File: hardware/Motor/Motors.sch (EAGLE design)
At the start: 34 parts, among them IC1 MC33269ST, Q1 BSS138, Q2 BSS138, U1 DRV8884PWPR, U2 PHOTON_WITH_HEADERS, U3 LS7083N-S

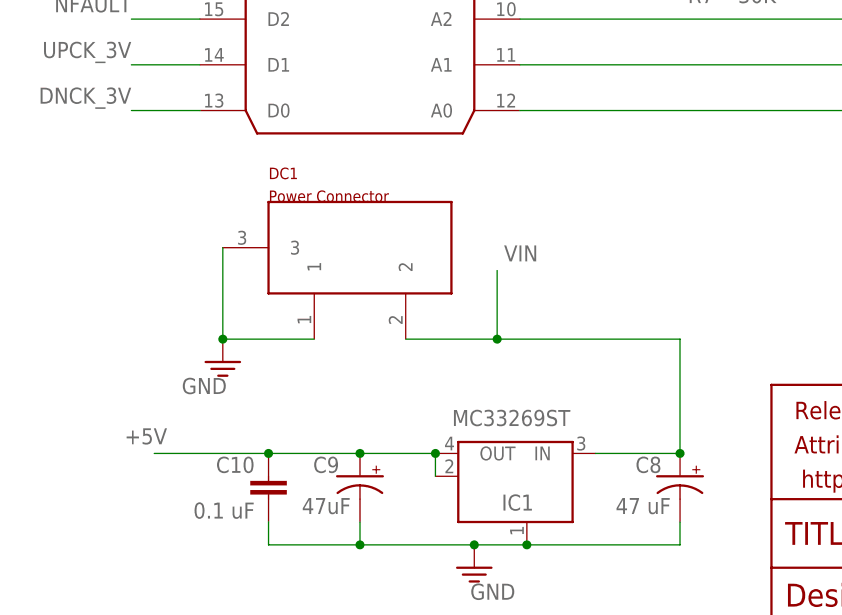
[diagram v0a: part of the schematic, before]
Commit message: Cumulative changes: adding light sources, boards, firmwares, construction details
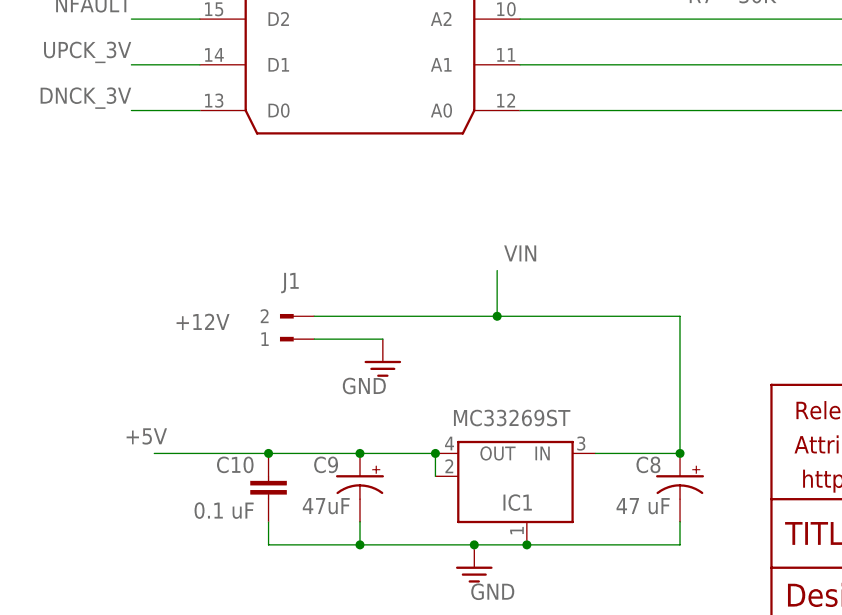
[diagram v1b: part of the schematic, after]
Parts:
- removed DC1: Power Connector, Spectron2:POWERSUPPLY_DC21MMX
- added J1: +12V, WEIDMULLER-PM5.08_2_90BLK:PM5.08/2/90BLK
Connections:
- net GND: now also J1.1; no longer DC1.1, DC1.3
- net VIN: now also J1.2; no longer DC1.2
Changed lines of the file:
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@@
 <?xml version="1.0" encoding="utf-8"?>
 <!DOCTYPE eagle SYSTEM "eagle.dtd">
-<eagle version="7.7.0">
+<eagle version="8.0.1">
 <drawing>
 <settings>
@@
 <layers>
 <layer number="1" name="Top" color="4" fill="1" visible="no" active="no"/>
+<layer number="2" name="Route2" color="1" fill="3" visible="no" active="no"/>
+<layer number="3" name="Route3" color="4" fill="3" visible="no" active="no"/>
+<layer number="4" name="Route4" color="1" fill="4" visible="no" active="no"/>
+<layer number="5" name="Route5" color="4" fill="4" visible="no" active="no"/>
+<layer number="6" name="Route6" color="1" fill="8" visible="no" active="no"/>
+<layer number="7" name="Route7" color="4" fill="8" visible="no" active="no"/>
+<layer number="8" name="Route8" color="1" fill="2" visible="no" active="no"/>
+<layer number="9" name="Route9" color="4" fill="2" visible="no" active="no"/>
+<layer number="10" name="Route10" color="1" fill="7" visible="no" active="no"/>
+<layer number="11" name="Route11" color="4" fill="7" visible="no" active="no"/>
+<layer number="12" name="Route12" color="1" fill="5" visible="no" active="no"/>
+<layer number="13" name="Route13" color="4" fill="5" visible="no" active="no"/>
+<layer number="14" name="Route14" color="1" fill="6" visible="no" active="no"/>
+<layer number="15" name="Route15" color="4" fill="6" visible="no" active="no"/>
 <layer number="16" name="Bottom" color="1" fill="1" visible="no" active="no"/>
 <layer number="17" name="Pads" color="2" fill="1" visible="no" active="no"/>
@@
 <part name="U2" library="Spectron2" deviceset="PHOTON" device="_WITH_HEADERS"/>
 <part name="U1" library="TI-DRV8884" deviceset="DRV8884PWPR" device=""/>
-<part name="DC1" library="Spectron2" deviceset="POWERSUPPLY_DC21MM" device="X" value="Power Connector"/>
 <part name="GND1" library="Spectron2" deviceset="GND" device=""/>
 <part name="GND6" library="Spectron2" deviceset="GND" device=""/>
@@
 <part name="GND10" library="Spectron2" deviceset="GND" device=""/>
 <part name="R7" library="Spectron2" deviceset="R-EU_" device="R0805" value="30K"/>
+<part name="J1" library="WEIDMULLER-PM5.08_2_90BLK" deviceset="PM5.08/2/90BLK" device="" value="+12V"/>
 </parts>
 <sheets>
@@
 <instance part="U2" gate="G$1" x="33.02" y="30.48" rot="MR0"/>
 <instance part="U1" gate="A" x="137.16" y="25.4"/>
-<instance part="DC1" gate="G$1" x="33.02" y="-12.7"/>
 <instance part="GND1" gate="1" x="119.38" y="2.54" rot="MR0"/>
-<instance part="GND6" gate="1" x="17.78" y="-25.4"/>
+<instance part="GND6" gate="1" x="35.56" y="-25.4"/>
 <instance part="IC1" gate="G$1" x="51.562" y="-40.64" smashed="yes" rot="MR0">
 <attribute name="NAME" x="52.324" y="-41.91" size="1.778" layer="95" rot="MR0"/>
@@
 <attribute name="VALUE" x="79.248" y="16.256" size="1.778" layer="96" rot="R180"/>
 </instance>
+<instance part="J1" gate="A" x="27.94" y="-22.86" smashed="yes" rot="R180">
+<attribute name="NAME" x="26.416" y="-15.494" size="1.778" layer="95" rot="R180"/>
+<attribute name="VALUE" x="18.542" y="-20.066" size="1.778" layer="96" rot="R180"/>
+</instance>
 </instances>
 <busses>
@@
 <net name="VIN" class="0">
 <segment>
-<wire x1="38.1" y1="-22.86" x2="48.26" y2="-22.86" width="0.1524" layer="91"/>
-<pinref part="DC1" gate="G$1" pin="2"/>
-<wire x1="48.26" y1="-22.86" x2="48.26" y2="-15.24" width="0.1524" layer="91"/>
+<wire x1="48.26" y1="-20.32" x2="48.26" y2="-15.24" width="0.1524" layer="91"/>
 <label x="49.022" y="-14.224" size="1.778" layer="95"/>
 <pinref part="IC1" gate="G$1" pin="IN"/>
 <pinref part="C8" gate="G$1" pin="+"/>
 <wire x1="68.58" y1="-35.56" x2="59.182" y2="-35.56" width="0.1524" layer="91"/>
-<wire x1="68.58" y1="-35.56" x2="68.58" y2="-22.86" width="0.1524" layer="91"/>
-<wire x1="68.58" y1="-22.86" x2="48.26" y2="-22.86" width="0.1524" layer="91"/>
+<wire x1="68.58" y1="-35.56" x2="68.58" y2="-20.32" width="0.1524" layer="91"/>
+<wire x1="68.58" y1="-20.32" x2="48.26" y2="-20.32" width="0.1524" layer="91"/>
 <junction x="68.58" y="-35.56"/>
-<junction x="48.26" y="-22.86"/>
+<junction x="48.26" y="-20.32"/>
+<pinref part="J1" gate="A" pin="2"/>
+<wire x1="27.94" y1="-20.32" x2="48.26" y2="-20.32" width="0.1524" layer="91"/>
 </segment>
 <segment>
@@
 </segment>
 <segment>
-<pinref part="DC1" gate="G$1" pin="3"/>
-<pinref part="DC1" gate="G$1" pin="1"/>
-<wire x1="17.78" y1="-12.7" x2="17.78" y2="-22.86" width="0.1524" layer="91"/>
-<pinref part="GND6" gate="1" pin="GND"/>
-<wire x1="17.78" y1="-22.86" x2="27.94" y2="-22.86" width="0.1524" layer="91"/>
-<junction x="17.78" y="-22.86"/>
-</segment>
-<segment>
 <pinref part="IC1" gate="G$1" pin="GND/ADJ"/>
 <pinref part="C8" gate="G$1" pin="-"/>
@@
 <wire x1="-45.72" y1="60.96" x2="-45.72" y2="68.58" width="0.1524" layer="91"/>
 </segment>
+<segment>
+<pinref part="GND6" gate="1" pin="GND"/>
+<pinref part="J1" gate="A" pin="1"/>
+<wire x1="35.56" y1="-22.86" x2="27.94" y2="-22.86" width="0.1524" layer="91"/>
+</segment>
 </net>
